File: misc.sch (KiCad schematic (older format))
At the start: 10 parts, among them J11 USB_OTG, U3 RT9193-28, U4 XC6206P302MR

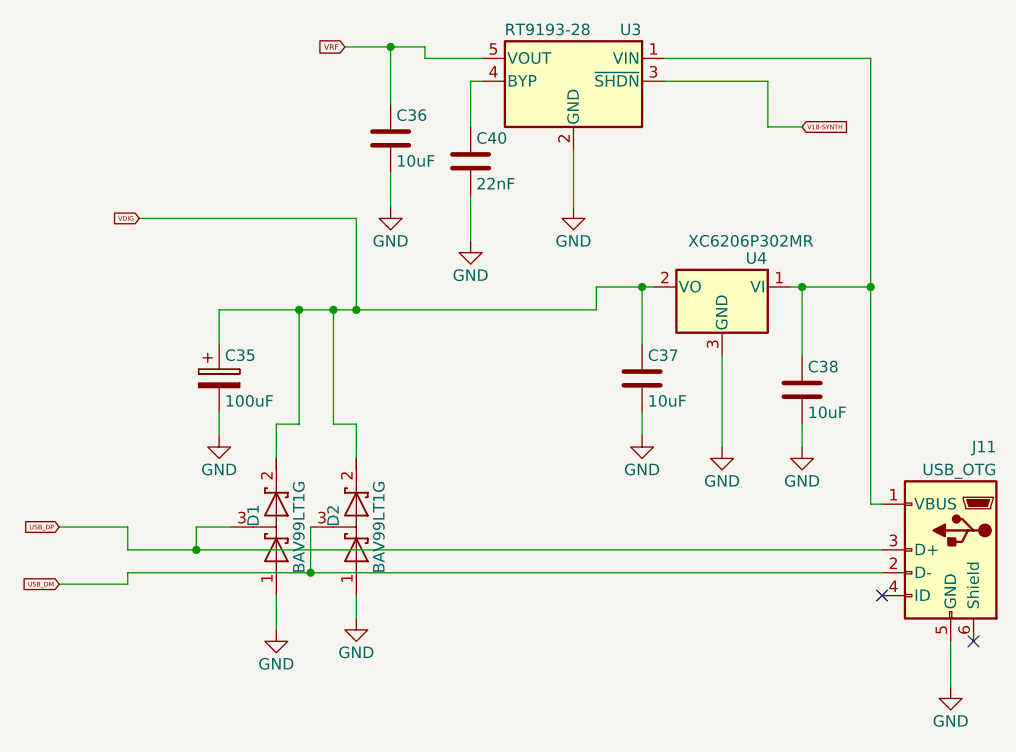
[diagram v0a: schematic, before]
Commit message: pcb version 2
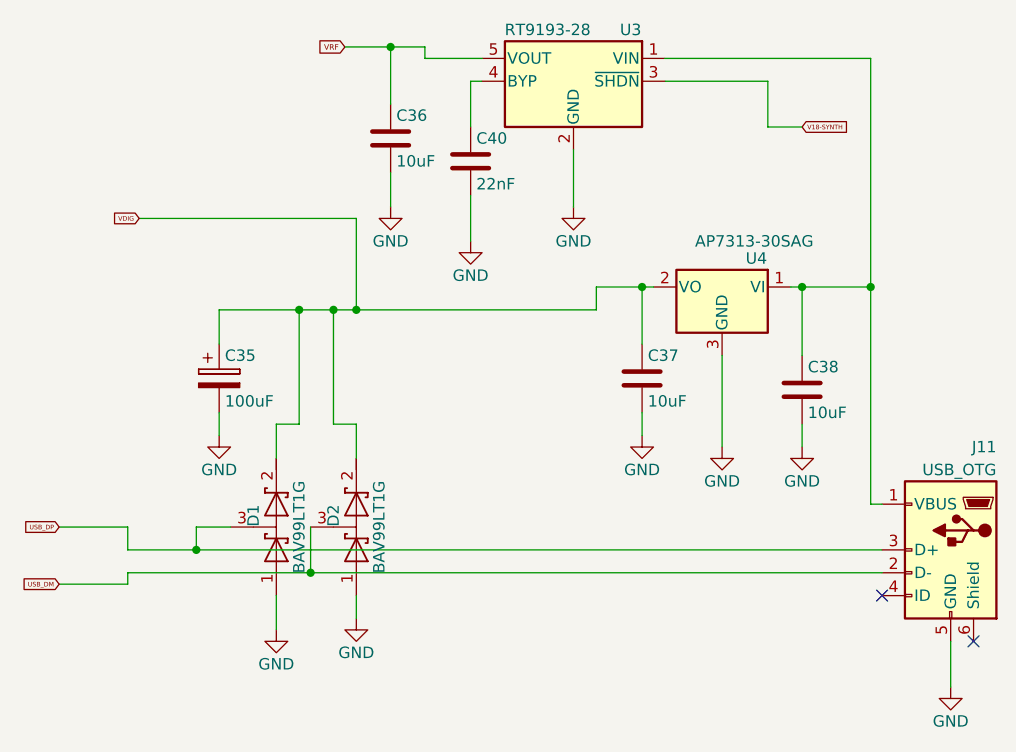
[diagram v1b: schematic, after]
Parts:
- U4: value XC6206P302MR -> AP7313-30SAG
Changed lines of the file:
@@
 P 6800 2550
 F 0 "U4" H 6650 2675 50  0000 C CNN
-F 1 "XC6206P302MR " H 6400 2750 50  0000 L CNN
+F 1 "AP7313-30SAG" H 6400 2750 50  0000 L CNN
 F 2 "TO_SOT_Packages_SMD:SOT-23" H 6800 2775 50  0001 C CIN
 F 3 "" H 6800 2500 50  0001 C CNN
